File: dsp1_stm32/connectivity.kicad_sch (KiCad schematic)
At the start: 54 parts, among them J1 Conn_01x04_Pin, J10 Conn_01x04_Socket, J11 Jack-DC, J12 AudioJack3, J13 Conn_01x04_Socket, J14 Conn_01x02_Pin, J15 Conn_01x02_Pin, J16 Conn_01x02_Pin, J17 Conn_01x02_Pin, J2 Conn_01x04_Pin, J3 Conn_01x04_Pin, J4 USB_C_Receptacle_USB2.0_14P, J5 AudioJack3, J6 AudioJack3, J7 AudioJack3, J8 Conn_01x04_Socket, J9 Conn_01x04_Socket, SW10 SW_Push, SW3 SW_SPDT, SW4 SW_SPDT, SW5 SW_SPDT, SW6 SW_SPDT, SW7 SW_Push, SW8 SW_Push, SW9 SW_Push, U11 USBLC6-2SC6, U12 USBLC6-2SC6, U13 USBLC6-2SC6, U14 USBLC6-2SC6, U2 USBLC6-2SC6, U3 USBLC6-2SC6, U4 USBLC6-2SC6, U5 USBLC6-2SC6, U6 USBLC6-2SC6, U7 USBLC6-2SC6, U8 WE-TVS-824015043

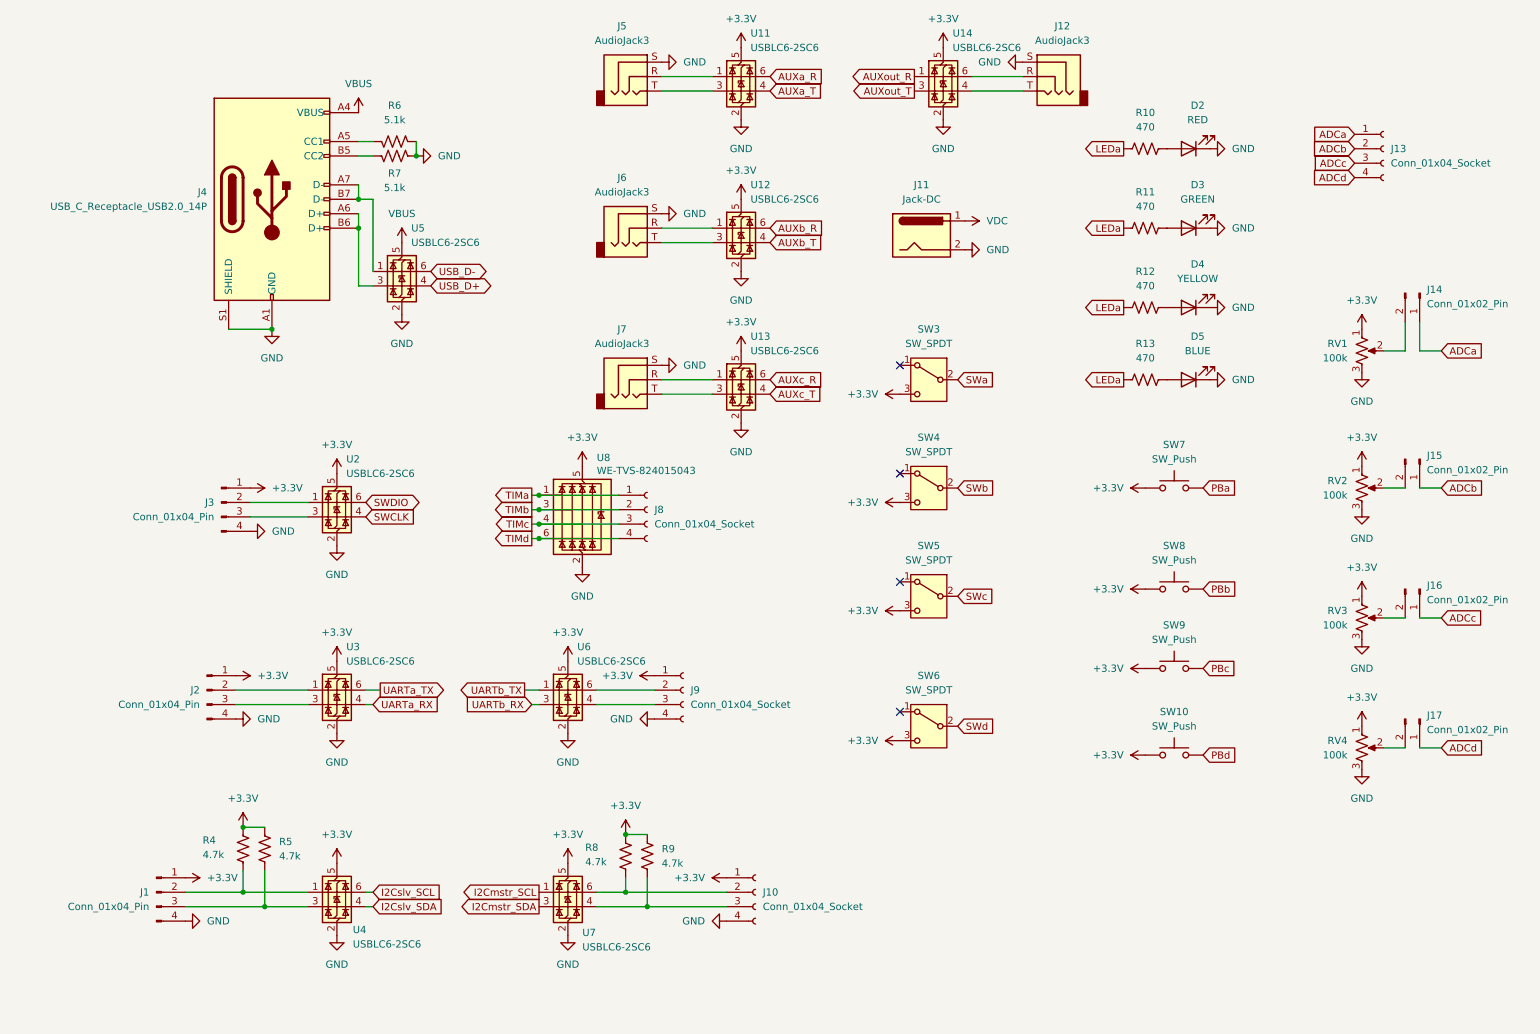
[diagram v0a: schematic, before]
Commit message: PCB dsp v1 done
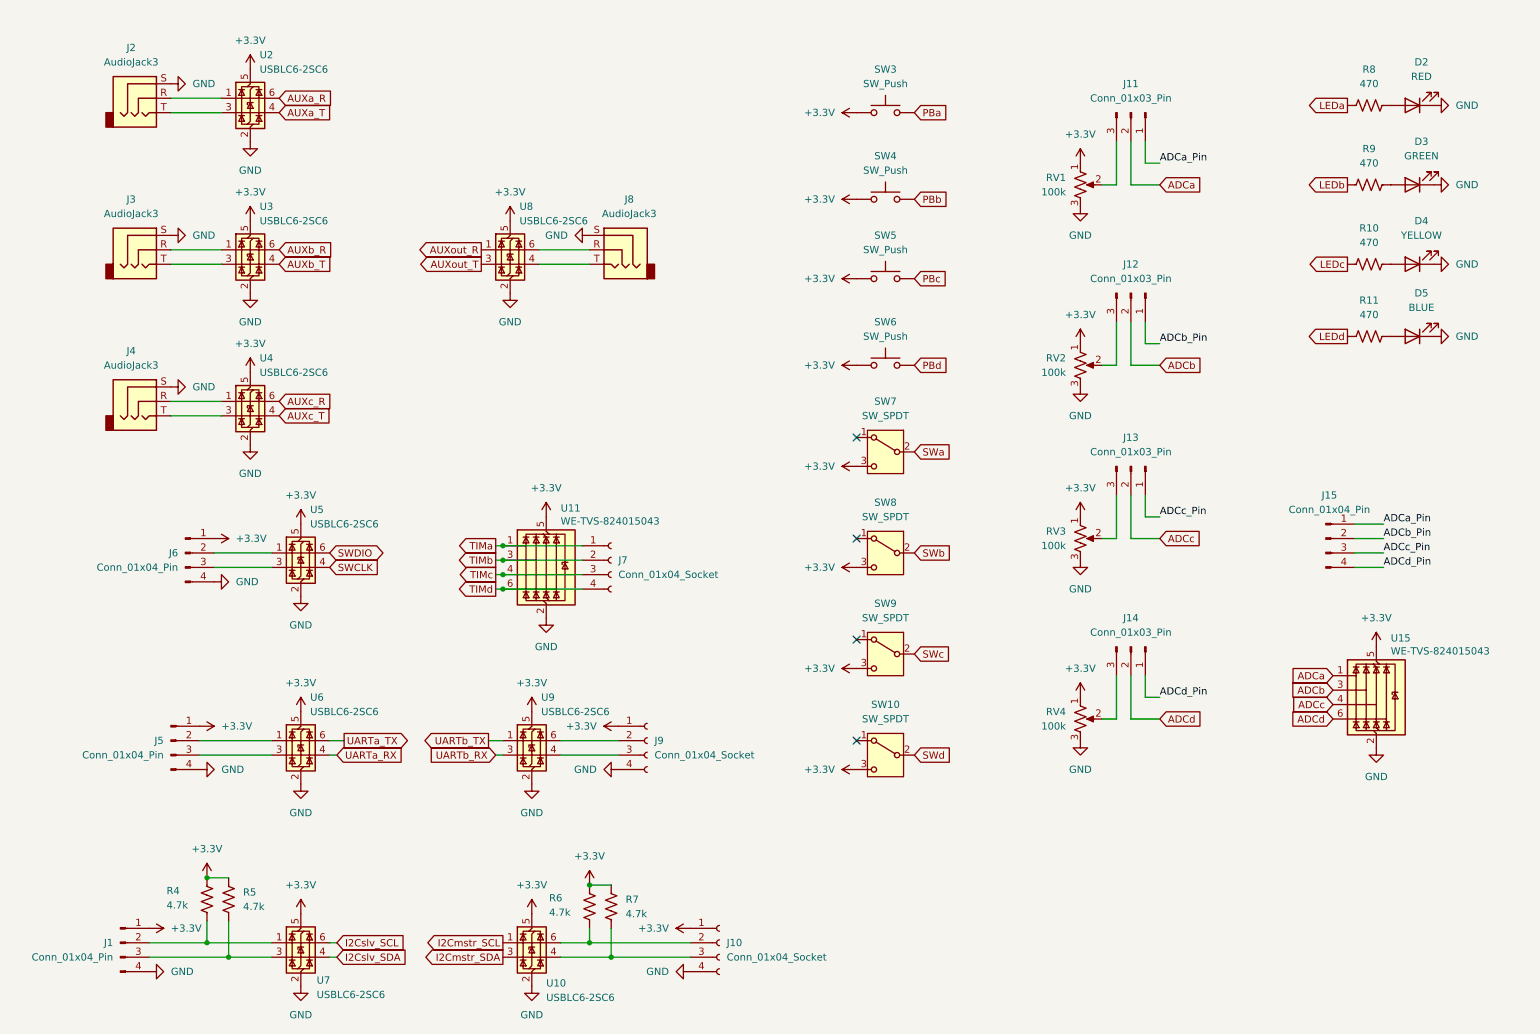
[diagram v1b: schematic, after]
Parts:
- removed J11: Jack-DC, Connector_BarrelJack:BarrelJack_SwitchcraftConxall_RAPC10U_Horizontal, symbol Connector:Jack-DC
- removed J13: Conn_01x04_Socket, Connector_PinSocket_2.54mm:PinSocket_1x04_P2.54mm_Vertical, symbol Connector:Conn_01x04_Socket
- removed J14, J15, J16, J17: Conn_01x02_Pin, Connector_PinHeader_2.54mm:PinHeader_1x02_P2.54mm_Vertical, symbol Connector:Conn_01x02_Pin
- removed J4: USB_C_Receptacle_USB2.0_14P, Connector_USB:USB_C_Receptacle_Palconn_UTC16-G, symbol Connector:USB_C_Receptacle_USB2.0_14P
- removed R6, R7: 5.1k, Resistor_SMD:R_0603_1608Metric, symbol Device:R_US
- removed U5: USBLC6-2SC6, Package_TO_SOT_SMD:SOT-23-6, symbol Power_Protection:USBLC6-2SC6
- added J11, J12, J13, J14: Conn_01x03_Pin, Connector_PinHeader_2.54mm:PinHeader_1x03_P2.54mm_Vertical, symbol Connector:Conn_01x03_Pin
- added J15: Conn_01x04_Pin, Connector_PinHeader_2.54mm:PinHeader_1x04_P2.54mm_Vertical, symbol Connector:Conn_01x04_Pin
- added U15: WE-TVS-824015043, Package_TO_SOT_SMD:SOT-23-6, symbol Power_Protection:WE-TVS-824015043
- SW10: renamed from SW6; footprint Button_Switch_SMD:Nidec_Copal_CAS-120A -> Button_Switch_SMD:SW_SPDT_PCM12
- SW3: renamed from SW7; footprint Button_Switch_SMD:SW_Push_1P1T_NO_CK_KMR2 -> Button_Switch_SMD:SW_SPST_PTS647_Sx38
- SW4: renamed from SW8; footprint Button_Switch_SMD:SW_Push_1P1T_NO_CK_KMR2 -> Button_Switch_SMD:SW_SPST_PTS647_Sx38
- SW5: renamed from SW9; footprint Button_Switch_SMD:SW_Push_1P1T_NO_CK_KMR2 -> Button_Switch_SMD:SW_SPST_PTS647_Sx38
- SW6: renamed from SW10; footprint Button_Switch_SMD:SW_Push_1P1T_NO_CK_KMR2 -> Button_Switch_SMD:SW_SPST_PTS647_Sx38
- SW7: renamed from SW3; footprint Button_Switch_SMD:Nidec_Copal_CAS-120A -> Button_Switch_SMD:SW_SPDT_PCM12
- SW8: renamed from SW4; footprint Button_Switch_SMD:Nidec_Copal_CAS-120A -> Button_Switch_SMD:SW_SPDT_PCM12
- SW9: renamed from SW5; footprint Button_Switch_SMD:Nidec_Copal_CAS-120A -> Button_Switch_SMD:SW_SPDT_PCM12
- renumbered J5 to J2, J6 to J3, J7 to J4, J2 to J5, J3 to J6, J8 to J7, J12 to J8, R12 to R10, R13 to R11, R8 to R6, R9 to R7, R10 to R8, R11 to R9, U7 to U10, U8 to U11, U11 to U2, U12 to U3, U13 to U4, U2 to U5, U3 to U6, U4 to U7, U14 to U8, U6 to U9
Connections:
- net +3.3V: now also U15.5 (VBUS)
- net ADCa: now also J11.2 (Pin_2), U15.1 (I/O1)
- net ADCb: now also J12.2 (Pin_2), U15.3 (I/O2)
- net ADCc: now also J13.2 (Pin_2), U15.4 (I/O3)
- net ADCd: now also J14.2 (Pin_2), U15.6 (I/O4)
- net GND: now also U15.2 (GND)
- net LEDa: no longer R10.1, R11.1, R9.1
- net at RV2.2: now also J12.3 (Pin_3)
- net at RV4.2: now also J14.3 (Pin_3)
- net at RV3.2: now also J13.3 (Pin_3)
- net at RV1.2: now also J11.3 (Pin_3)
- new net ADCa_Pin: J11.1 (Pin_1), J15.1 (Pin_1)
- new net ADCb_Pin: J12.1 (Pin_1), J15.2 (Pin_2)
- new net ADCc_Pin: J13.1 (Pin_1), J15.3 (Pin_3)
- new net ADCd_Pin: J14.1 (Pin_1), J15.4 (Pin_4)
- new net LEDb: R9.1
- new net LEDc: R10.1
- new net LEDd: R11.1
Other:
- moved on the sheet: D2, D3, D4, D5, J1, J10, J2, J3, J4, J5, J6, J7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
